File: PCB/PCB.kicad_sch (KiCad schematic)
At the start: 14 parts, among them J1 USB_C_Receptacle_USB2.0_14P, U1 CH552G, U2 AMS1117-3.3, U3 W25Q128JVSIQTR, U4 PAM8302AADCR

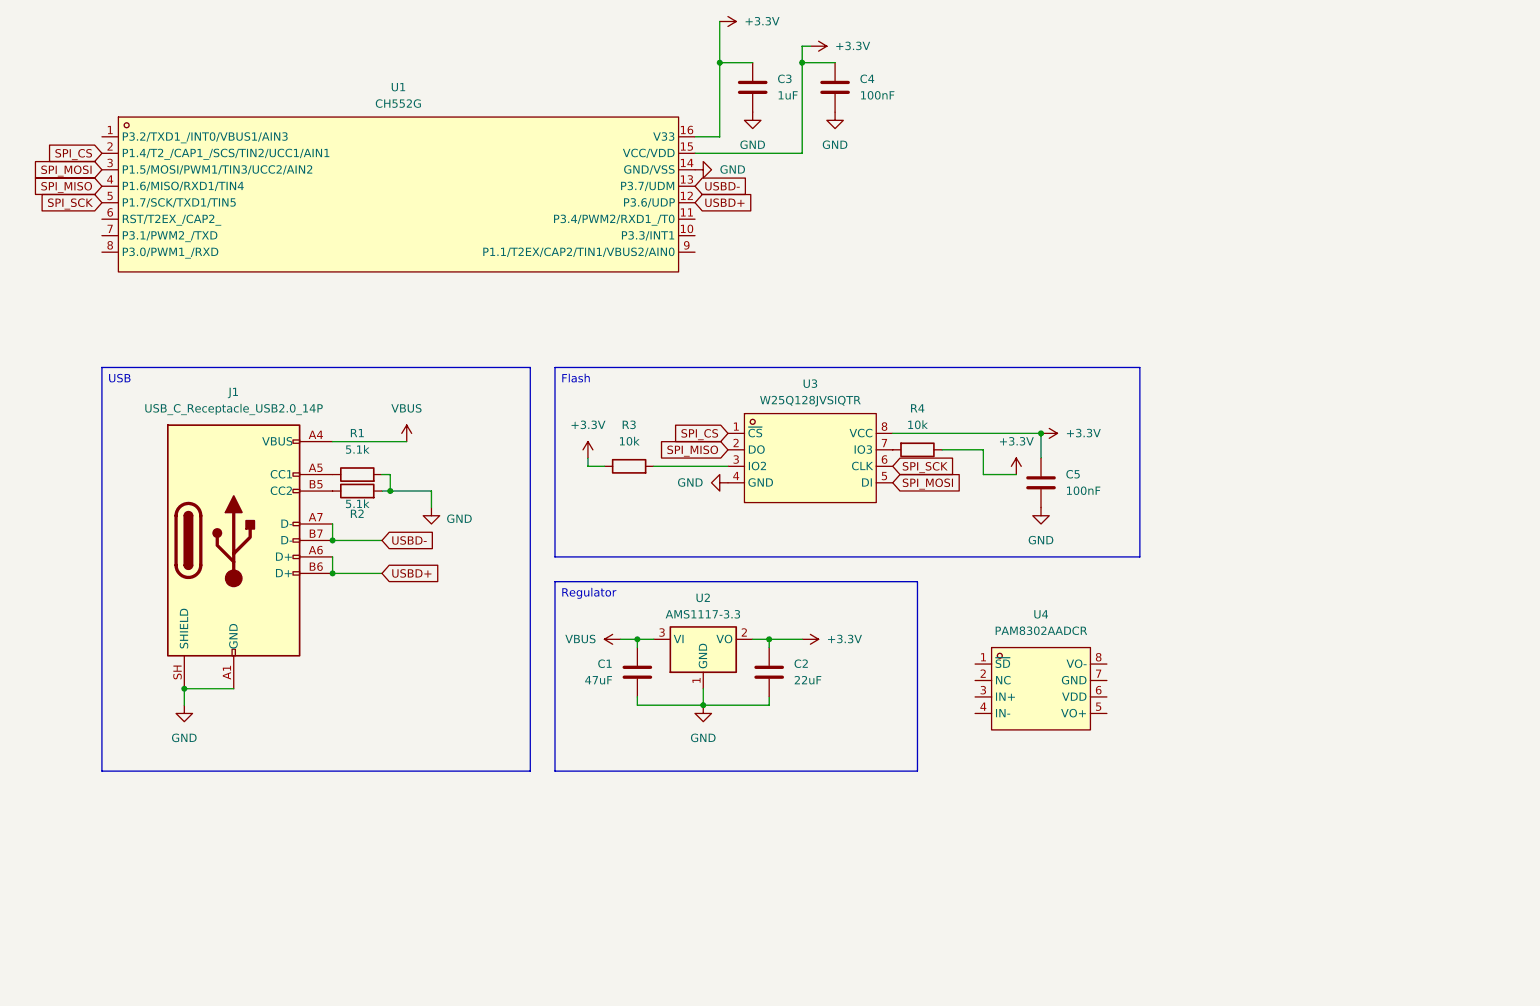
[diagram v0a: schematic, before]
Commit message: igb
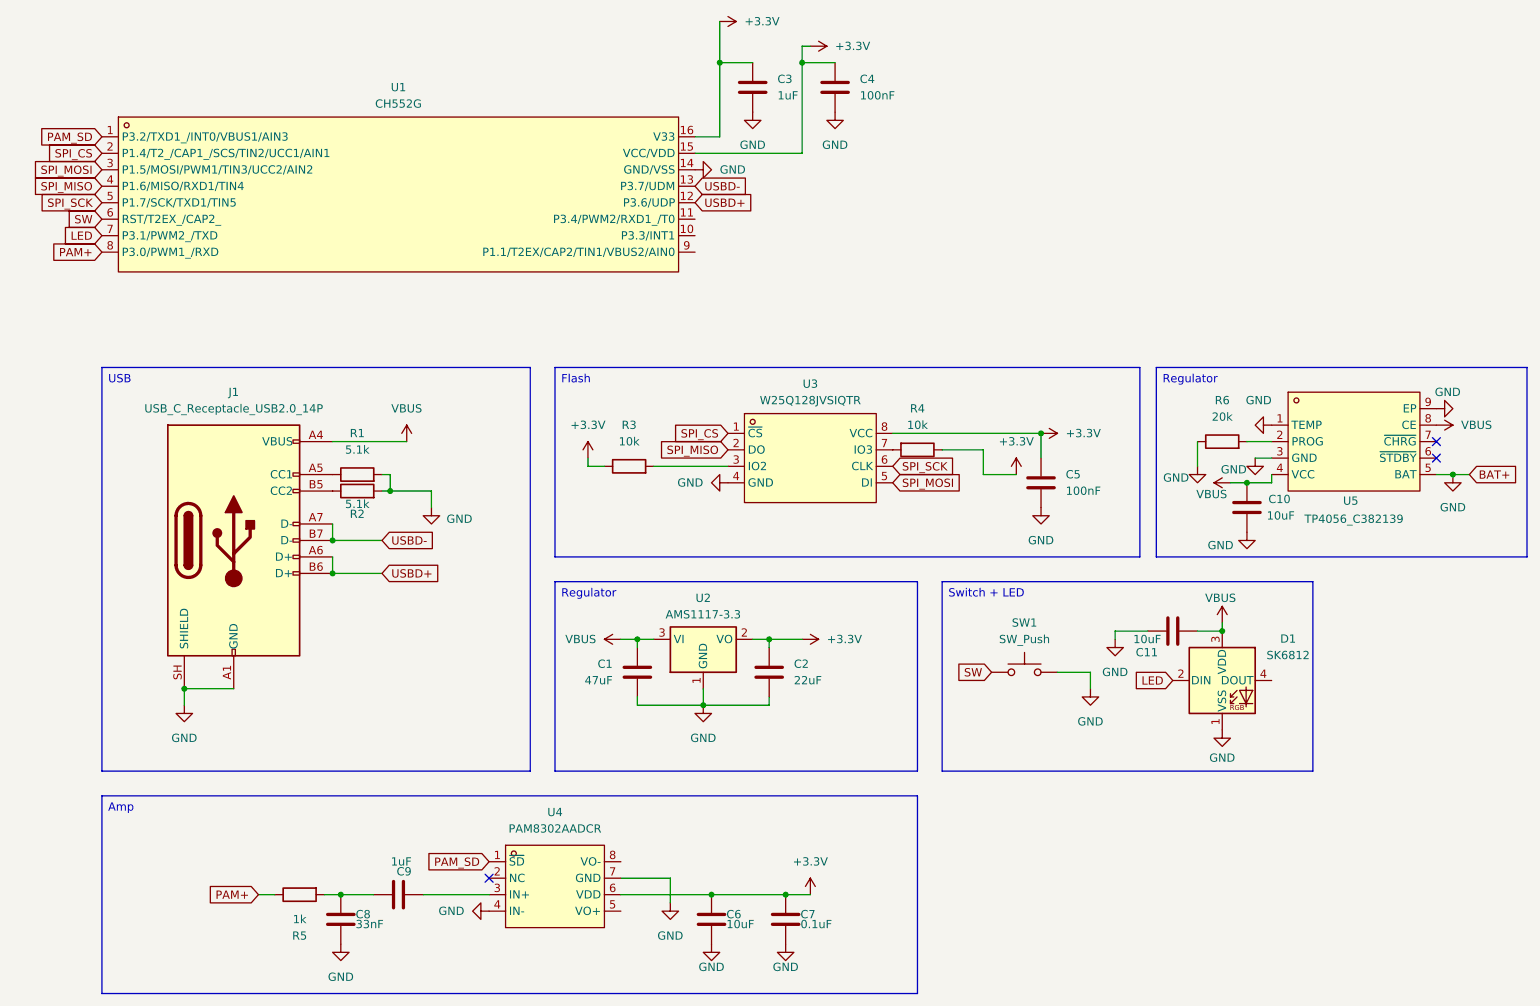
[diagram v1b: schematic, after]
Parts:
- added C10, C11, C6: 10uF, symbol Device:C
- added C7: 0.1uF, symbol Device:C
- added C8: 33nF, symbol Device:C
- added C9: 1uF, symbol Device:C
- added D1: SK6812, LED_SMD:LED_SK6812_PLCC4_5.0x5.0mm_P3.2mm, symbol LED:SK6812
- added R5: 1k, symbol Device:R
- added R6: 20k, symbol Device:R
- added SW1: SW_Push, Capacitor_SMD:C_0201_0603Metric, symbol Switch:SW_Push
- added U5: TP4056_C382139, easyeda2kicad:ESOP-8_L4.9-W3.9-P1.27-LS6.0-BL-EP, symbol burrito:TP4056_C382139
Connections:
- net +3.3V: now also U4.6 (VDD), C6.2, C7.2
- net GND: now also U4.4 (IN-), U4.7 (GND), C10.2, C11.1, C6.1, C7.1, C8.1, D1.1 (VSS), R6.1, SW1.2, U5.1 (TEMP), U5.3 (GND), U5.5 (BAT), U5.9 (EP)
- net VBUS: now also C10.1, C11.2, D1.3 (VDD), U5.4 (VCC), U5.8 (CE)
- net PAM_SD: now reaches U4.1 (~{SD})
- net PAM_SD: now also U1.1 (P3.2/TXD1_/INT0/VBUS1/AIN3)
- net at U4.3 (IN+): now also C9.1
- net SW: now reaches U1.6 (RST/T2EX_/CAP2_)
- net SW: now also SW1.1
- net LED: now reaches U1.7 (P3.1/PWM2_/TXD)
- net LED: now also D1.2 (DIN)
- net PAM+: now reaches U1.8 (P3.0/PWM1_/RXD)
- net PAM+: now also R5.1
- new net: C8.2, C9.2, R5.2
- new net: R6.2, U5.2 (PROG)
- no-connect marks 0 -> 3
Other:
- moved on the sheet: U4
